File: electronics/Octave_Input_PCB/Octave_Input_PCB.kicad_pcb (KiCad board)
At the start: 2 copper layers, 87.8 x 95.8 mm, 66 parts, among them J1 HRO_TYPE-C-31-M-12, SW1 SW_Hot_Swap_Socket, SW10 SW_Hot_Swap_Socket, SW11 SW_Hot_Swap_Socket, SW12 SW_Hot_Swap_Socket, SW13 SW_Hot_Swap_Socket, SW14 Alps_Alpine_RKJXV1224, SW15 Bourns_PEC12R-4xxxF-Sxxx, SW2 SW_Hot_Swap_Socket, SW21 Alps_Alpine_SKRP, SW22 Alps_Alpine_SKRP, SW3 SW_Hot_Swap_Socket, SW4 SW_Hot_Swap_Socket, SW5 SW_Hot_Swap_Socket, SW6 SW_Hot_Swap_Socket, SW7 SW_Hot_Swap_Socket, SW8 SW_Hot_Swap_Socket, SW9 SW_Hot_Swap_Socket, U1 AP2112K-3.3, U2 Raspberry_Pi_RP2040, U3 W25Q64JVSS, Y1 12MHz

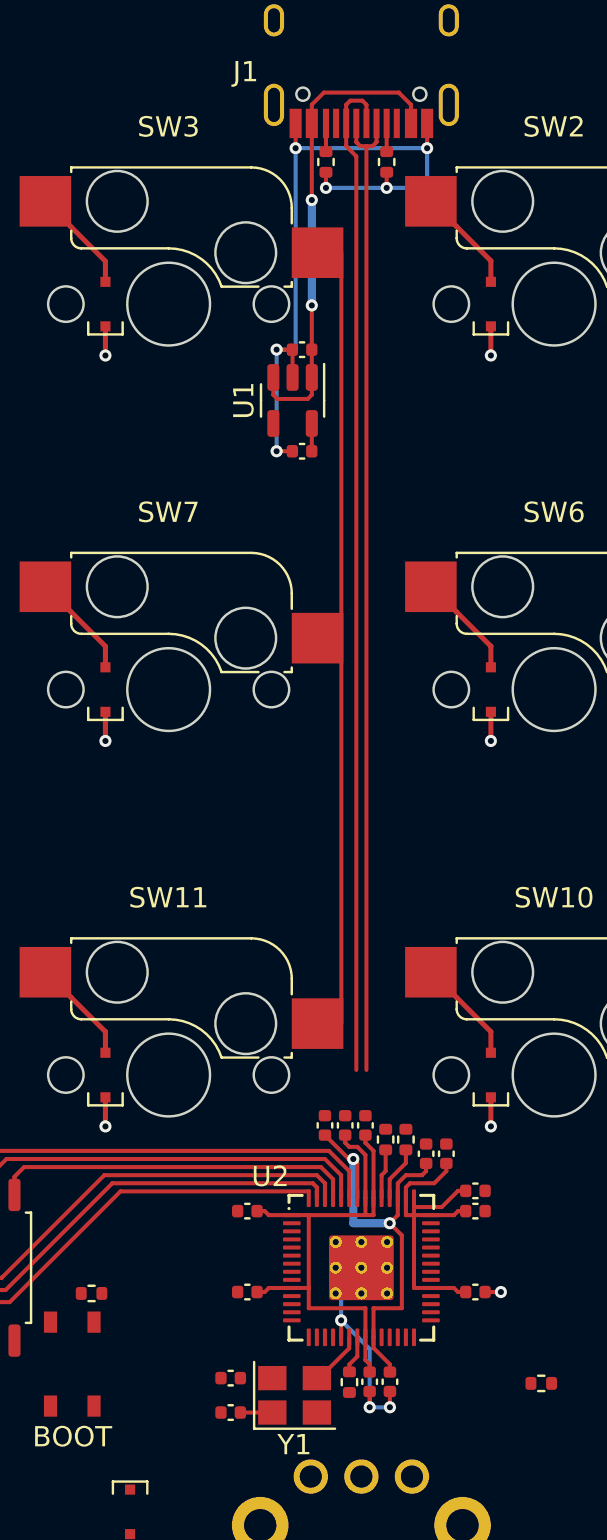
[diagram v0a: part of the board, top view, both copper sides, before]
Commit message: [WIP] Update PCB
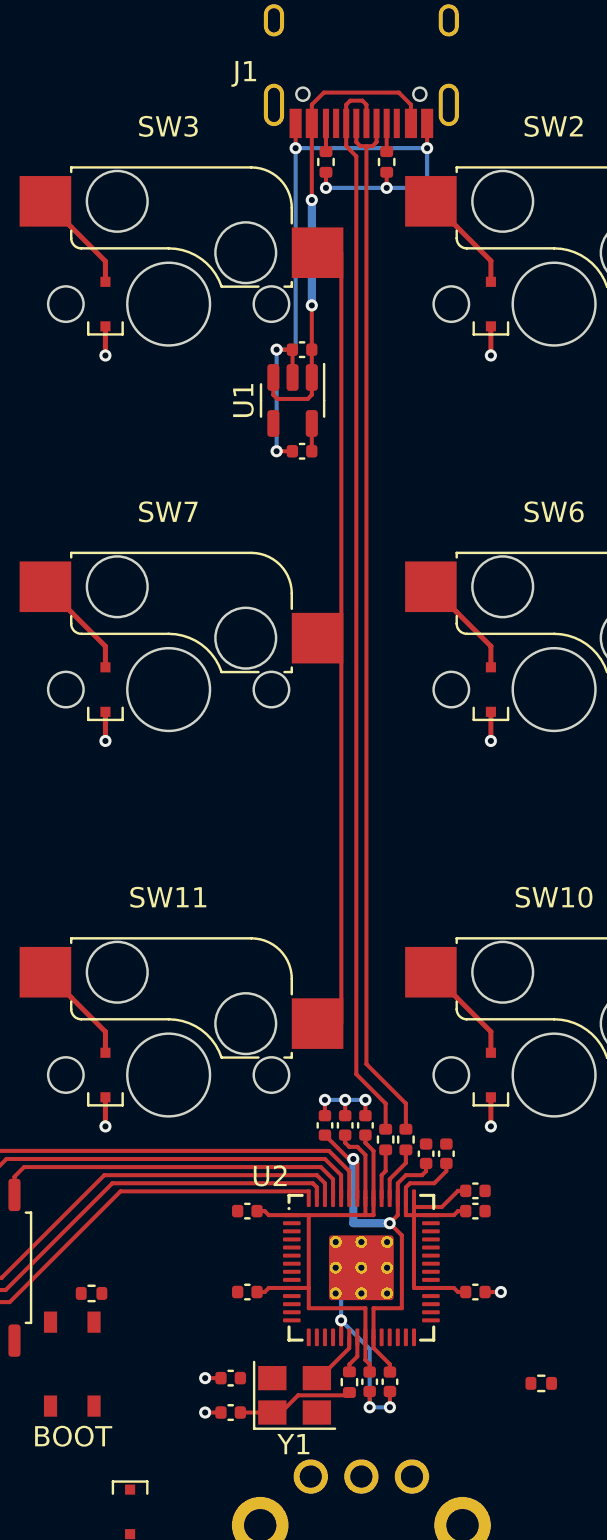
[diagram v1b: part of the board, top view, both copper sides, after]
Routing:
- net GND: track 46.8 -> 52.7 mm, vias 10 -> 15
- net Net-(C16-Pad1): track 1.58 -> 6.03 mm
- net Net-(J1-PadA7): track 48.7 -> 52.4 mm
- net Net-(J1-PadA6): track 50.0 -> 53.5 mm
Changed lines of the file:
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@@
   (title_block
     (title "Octave - Input PCB")
-    (date "2022-05-21")
+    (date "2022-05-23")
     (rev "5.a")
     (comment 4 "https://github.com/takayoshiotake/octave-12-key-macropad")
@@
       (effects (font (size 1 1) (thickness 0.15)))
     )
-    (fp_rect (start -2.8 -1.8) (end 2.8 1.8) (layer "Margin") (width 0.05) (fill none))
+    (fp_rect (start -2.8 -1.8) (end 2.8 1.8) (layer "F.CrtYd") (width 0.05) (fill none))
     (fp_line (start -0.4 1.1) (end 0.4 1.1) (layer "F.Fab") (width 0.1))
     (fp_line (start -0.4 -1.1) (end 0.4 -1.1) (layer "F.Fab") (width 0.1))
     (fp_rect (start -2.1 -1.6) (end 2.1 1.6) (layer "F.Fab") (width 0.1) (fill none))
-    (fp_arc (start 0.4 -1.1) (mid 1.5 0) (end 0.4 1.1) (layer "F.Fab") (width 0.1))
     (fp_arc (start -0.4 1.1) (mid -1.5 0) (end -0.4 -1.1) (layer "F.Fab") (width 0.1))
+    (fp_arc (start 0.4 -1.1) (mid 1.5 0) (end 0.4 1.1) (layer "F.Fab") (width 0.1))
     (pad "1" smd rect (at -2.075 -1.075 90) (size 1.05 0.65) (layers "F.Cu" "F.Paste" "F.Mask")
       (net 28 "GND") (pinfunction "1") (pintype "passive"))
@@
       (effects (font (size 1 1) (thickness 0.15)))
     )
-    (fp_rect (start -2.8 -1.8) (end 2.8 1.8) (layer "Margin") (width 0.05) (fill none))
-    (fp_line (start -0.4 1.1) (end 0.4 1.1) (layer "F.Fab") (width 0.1))
+    (fp_rect (start -2.8 -1.8) (end 2.8 1.8) (layer "F.CrtYd") (width 0.05) (fill none))
     (fp_line (start -0.4 -1.1) (end 0.4 -1.1) (layer "F.Fab") (width 0.1))
+    (fp_line (start -0.4 1.1) (end 0.4 1.1) (layer "F.Fab") (width 0.1))
     (fp_rect (start -2.1 -1.6) (end 2.1 1.6) (layer "F.Fab") (width 0.1) (fill none))
     (fp_arc (start 0.4 -1.1) (mid 1.5 0) (end 0.4 1.1) (layer "F.Fab") (width 0.1))
@@
     )
   )
-  (footprint "Crystal:Crystal_SMD_3225-4Pin_3.2x2.5mm" locked (layer "F.Cu")
+  (footprint "Crystal:Crystal_SMD_3225-4Pin_3.2x2.5mm" (layer "F.Cu")
     (at 82.425 111.08)
     (descr "SMD Crystal SERIES SMD3225/4 http://www.txccrystal.com/images/pdf/7m-accuracy.pdf, 3.2x2.5mm^2 package")
@@
   (segment (start 111.1758 112.1858) (end 111.1758 113.25) (width 0.25) (layer "F.Cu") (net 25))
   (segment (start 82.3125 59.4) (end 82.315 59.4025) (width 0.2) (layer "F.Cu") (net 28))
+  (segment (start 83.925 97.26) (end 83.925 96.48) (width 0.2) (layer "F.Cu") (net 28))
   (segment (start 91.84 105.975) (end 92.619999 105.975) (width 0.2) (layer "F.Cu") (net 28))
   (segment (start 88.975 48.2205) (end 88.975 49.445499) (width 0.2) (layer "F.Cu") (net 28))
@@
   (segment (start 81.535 59.4) (end 82.3125 59.4) (width 0.2) (layer "F.Cu") (net 28))
   (segment (start 83.975 50.6355) (end 83.975 51.4055) (width 0.2) (layer "F.Cu") (net 28))
+  (segment (start 85.925 96.48) (end 85.925 97.26) (width 0.2) (layer "F.Cu") (net 28))
   (segment (start 87.135 110.89) (end 87.135 111.669999) (width 0.2) (layer "F.Cu") (net 28))
   (segment (start 81.535 64.4225) (end 82.315 64.4225) (width 0.2) (layer "F.Cu") (net 28))
+  (segment (start 78.005 111.93) (end 78.785 111.93) (width 0.2) (layer "F.Cu") (net 28))
+  (segment (start 78.785 110.23) (end 78.005 110.23) (width 0.2) (layer "F.Cu") (net 28))
   (segment (start 86.975 50.6355) (end 86.975 51.4055) (width 0.2) (layer "F.Cu") (net 28))
   (segment (start 82.325 60.775) (end 82.325 59.4125) (width 0.2) (layer "F.Cu") (net 28))
   (segment (start 86.135 110.89) (end 86.135 111.669999) (width 0.2) (layer "F.Cu") (net 28))
   (segment (start 82.475 49.445499) (end 82.475 48.2205) (width 0.2) (layer "F.Cu") (net 28))
+  (segment (start 84.925 97.26) (end 84.925 96.48) (width 0.2) (layer "F.Cu") (net 28))
+  (via (at 83.925 96.48) (size 0.6) (drill 0.3) (layers "F.Cu" "B.Cu") (remove_unused_layers) (keep_end_layers) (net 28))
+  (via (at 78.005 111.93) (size 0.6) (drill 0.3) (layers "F.Cu" "B.Cu") (remove_unused_layers) (keep_end_layers) (net 28))
   (via (at 83.975 51.4055) (size 0.6) (drill 0.3) (layers "F.Cu" "B.Cu") (remove_unused_layers) (keep_end_layers) (net 28))
+  (via (at 84.925 96.48) (size 0.6) (drill 0.3) (layers "F.Cu" "B.Cu") (remove_unused_layers) (keep_end_layers) (net 28))
   (via (at 87.135 111.669999) (size 0.6) (drill 0.3) (layers "F.Cu" "B.Cu") (remove_unused_layers) (keep_end_layers) (net 28))
   (via (at 81.535 64.4225) (size 0.6) (drill 0.3) (layers "F.Cu" "B.Cu") (remove_unused_layers) (keep_end_layers) (net 28))
   (via (at 92.619999 105.975) (size 0.6) (drill 0.3) (layers "F.Cu" "B.Cu") (remove_unused_layers) (keep_end_layers) (net 28))
   (via (at 88.975 49.445499) (size 0.6) (drill 0.3) (layers "F.Cu" "B.Cu") (remove_unused_layers) (keep_end_layers) (net 28))
+  (via (at 85.925 96.48) (size 0.6) (drill 0.3) (layers "F.Cu" "B.Cu") (remove_unused_layers) (keep_end_layers) (net 28))
   (via (at 86.135 111.669999) (size 0.6) (drill 0.3) (layers "F.Cu" "B.Cu") (remove_unused_layers) (keep_end_layers) (net 28))
+  (via (at 78.005 110.23) (size 0.6) (drill 0.3) (layers "F.Cu" "B.Cu") (remove_unused_layers) (keep_end_layers) (net 28))
   (via (at 84.725 107.375) (size 0.6) (drill 0.3) (layers "F.Cu" "B.Cu") (remove_unused_layers) (keep_end_layers) (net 28))
   (via (at 81.535 59.4) (size 0.6) (drill 0.3) (layers "F.Cu" "B.Cu") (remove_unused_layers) (keep_end_layers) (net 28))
@@
   (segment (start 82.475 49.445499) (end 83.954501 49.445499) (width 0.2) (layer "B.Cu") (net 28))
   (segment (start 84.725 107.375) (end 84.725 106.315) (width 0.2) (layer "B.Cu") (net 28))
+  (segment (start 85.925 96.48) (end 83.925 96.48) (width 0.2) (layer "B.Cu") (net 28))
   (segment (start 81.535 59.4) (end 82.475 59.4) (width 0.2) (layer "B.Cu") (net 28))
   (segment (start 83.975 51.4055) (end 86.975 51.4055) (width 0.2) (layer "B.Cu") (net 28))
@@
   (segment (start 81.535 59.4) (end 81.535 64.4225) (width 0.2) (layer "B.Cu") (net 28))
   (segment (start 86.975 49.6155) (end 86.975 48.2205) (width 0.2) (layer "F.Cu") (net 32))
+  (segment (start 86.925 97.93) (end 86.925 96.66) (width 0.2) (layer "F.Cu") (net 33))
   (segment (start 85.175 47.0955) (end 84.975 47.2955) (width 0.2) (layer "F.Cu") (net 33))
-  (segment (start 85.475 49.8455) (end 85.475 95) (width 0.2) (layer "F.Cu") (net 33))
+  (segment (start 86.925 96.66) (end 85.475 95.21) (width 0.2) (layer "F.Cu") (net 33))
   (segment (start 85.775 47.0955) (end 85.975 47.2955) (width 0.2) (layer "F.Cu") (net 33))
   (segment (start 85.775 47.0955) (end 85.175 47.0955) (width 0.2) (layer "F.Cu") (net 33))
-  (segment (start 84.975 48.2205) (end 84.975 49.3455) (width 0.2) (layer "F.Cu") (net 33))
   (segment (start 84.975 48.2205) (end 84.975 47.2955) (width 0.2) (layer "F.Cu") (net 33))
+  (segment (start 85.475 95.21) (end 85.475 49.8455) (width 0.2) (layer "F.Cu") (net 33))
   (segment (start 85.975 47.2955) (end 85.975 48.2205) (width 0.2) (layer "F.Cu") (net 33))
-  (segment (start 84.975 49.3455) (end 85.475 49.8455) (width 0.2) (layer "F.Cu") (net 33))
+  (segment (start 85.475 49.8455) (end 84.975 49.3455) (width 0.2) (layer "F.Cu") (net 33))
+  (segment (start 84.975 49.3455) (end 84.975 48.2205) (width 0.2) (layer "F.Cu") (net 33))
   (segment (start 85.475 49.1455) (end 85.475 48.2205) (width 0.2) (layer "F.Cu") (net 35))
   (segment (start 85.675 49.3455) (end 86.275 49.3455) (width 0.2) (layer "F.Cu") (net 35))
+  (segment (start 85.975 49.3455) (end 85.975 94.71) (width 0.2) (layer "F.Cu") (net 35))
   (segment (start 85.675 49.3455) (end 85.475 49.1455) (width 0.2) (layer "F.Cu") (net 35))
+  (segment (start 87.925 96.66) (end 87.925 97.93) (width 0.2) (layer "F.Cu") (net 35))
   (segment (start 86.475 48.2205) (end 86.475 49.1455) (width 0.2) (layer "F.Cu") (net 35))
+  (segment (start 85.975 94.71) (end 87.925 96.66) (width 0.2) (layer "F.Cu") (net 35))
   (segment (start 86.275 49.3455) (end 86.475 49.1455) (width 0.2) (layer "F.Cu") (net 35))
-  (segment (start 85.975 95) (end 85.975 49.3455) (width 0.2) (layer "F.Cu") (net 35))
   (segment (start 83.975 49.6155) (end 83.975 48.2205) (width 0.2) (layer "F.Cu") (net 36))
   (segment (start 86.325 108.74) (end 86.325 108.2125) (width 0.2) (layer "F.Cu") (net 38))
@@
   (segment (start 83.525 110.23) (end 83.645 110.23) (width 0.2) (layer "F.Cu") (net 83))
   (segment (start 85.125 108.2125) (end 85.125 108.75) (width 0.2) (layer "F.Cu") (net 83))
+  (segment (start 82.6 111.08) (end 81.75 111.93) (width 0.2) (layer "F.Cu") (net 84))
+  (segment (start 82.6 111.08) (end 84.995 111.08) (width 0.2) (layer "F.Cu") (net 84))
+  (segment (start 81.75 111.93) (end 81.325 111.93) (width 0.2) (layer "F.Cu") (net 84))
+  (segment (start 84.995 111.08) (end 85.135 110.94) (width 0.2) (layer "F.Cu") (net 84))
+  (segment (start 85.135 110.94) (end 84.971511 111.103489) (width 0.2) (layer "F.Cu") (net 84))
   (segment (start 81.325 111.93) (end 79.745 111.93) (width 0.2) (layer "F.Cu") (net 84))
   (segment (start 85.135 109.92) (end 85.135 109.55) (width 0.2) (layer "F.Cu") (net 85))
@@
     (connect_pads (clearance 0))
     (min_thickness 0.254) (filled_areas_thickness no)
-    (fill (thermal_gap 0.508) (thermal_bridge_width 0.508))
+    (fill yes (thermal_gap 0.508) (thermal_bridge_width 0.508))
     (polygon
       (pts
